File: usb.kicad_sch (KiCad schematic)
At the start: 29 parts, among them J3 USB_C_Receptacle_USB2.0_16P, U2 NCP730BMT330, U3 FT230X, U4 TPD4E05U06QDQARQ1

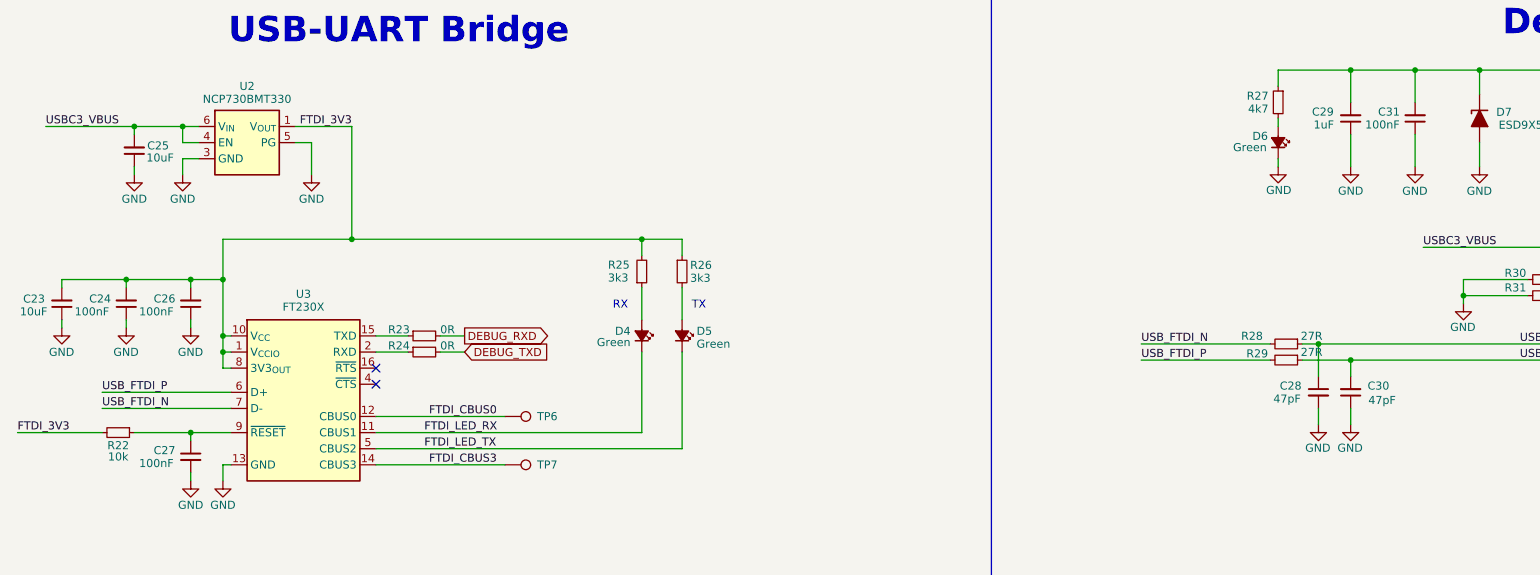
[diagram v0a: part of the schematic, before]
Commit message: Final BOM changes, gerbers
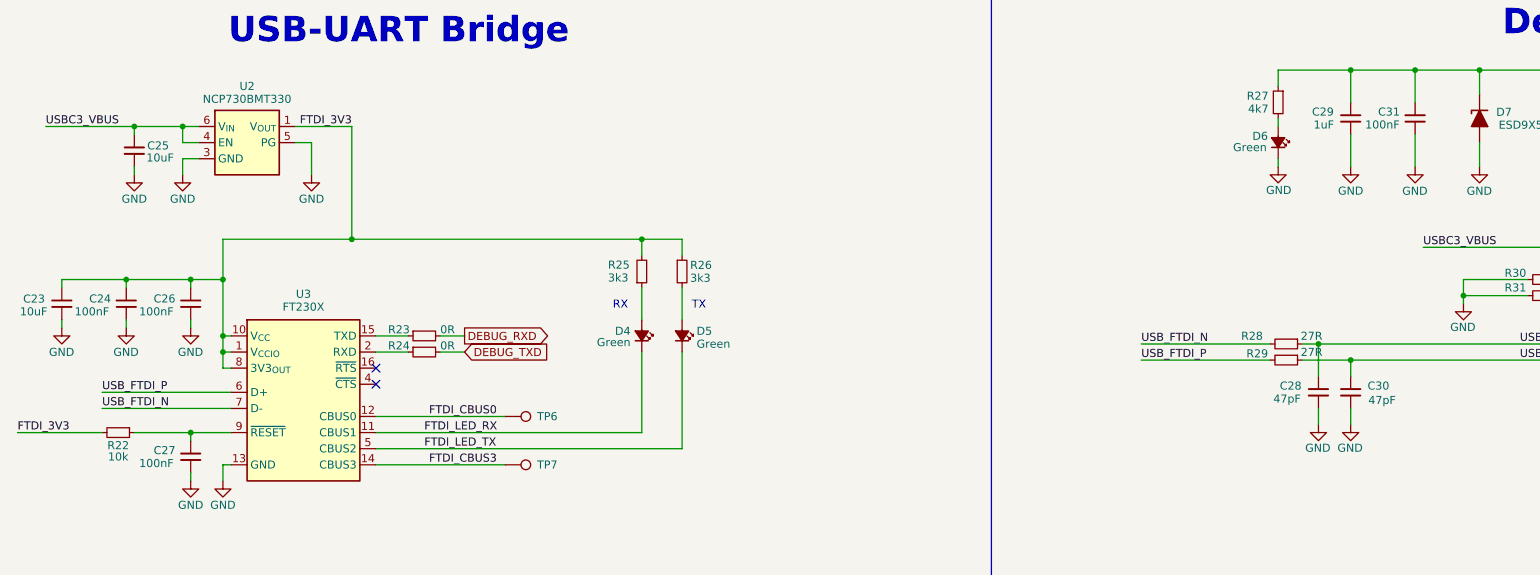
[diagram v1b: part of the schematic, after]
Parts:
- C23, C25: LCSC (none) -> C96446
- C24, C26, C27, C31: LCSC (none) -> C14663
- C28, C30: LCSC (none) -> C1567
- C29: LCSC (none) -> C15849
- D4, D5: LCSC (none) -> C2290
- D6: LCSC (none) -> C12065
- D7: LCSC (none) -> C87910
- J3: LCSC (none) -> C3020560
- R22: LCSC (none) -> C25804
- R23, R24: LCSC (none) -> C17168
- R25, R26: LCSC (none) -> C22978
- R27: LCSC (none) -> C23162
- R28, R29: LCSC (none) -> C227752
- R30, R31: LCSC (none) -> C23186
- U2: LCSC (none) -> C892821
- U3: LCSC (none) -> C128629
- U4: LCSC (none) -> C81353
